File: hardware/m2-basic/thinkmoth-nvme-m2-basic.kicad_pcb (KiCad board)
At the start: 4 copper layers, 31 x 68.4 mm, 24 parts, among them J1 ExpressCard, J2 MDT180M03001, J3 TF-001B, U1 GL823K-HCY04

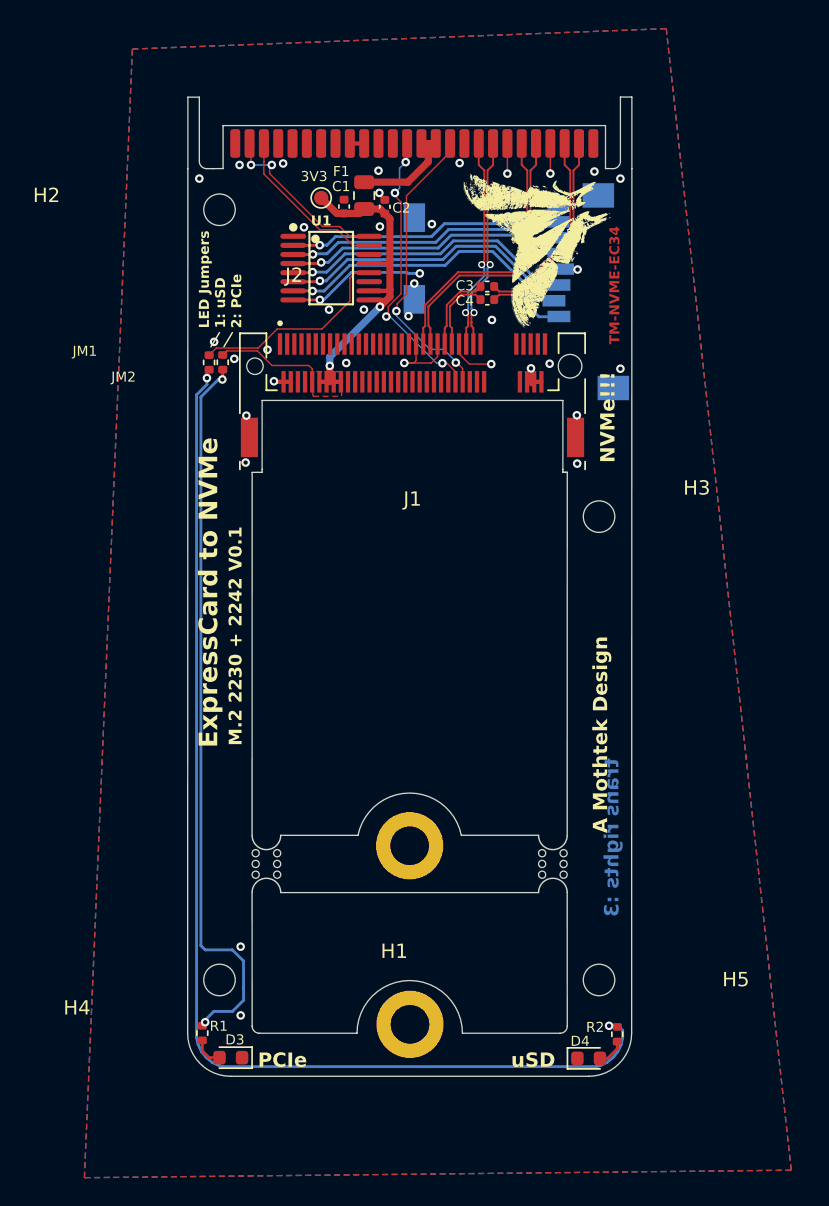
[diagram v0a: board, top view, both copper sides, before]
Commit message: minor tweaks
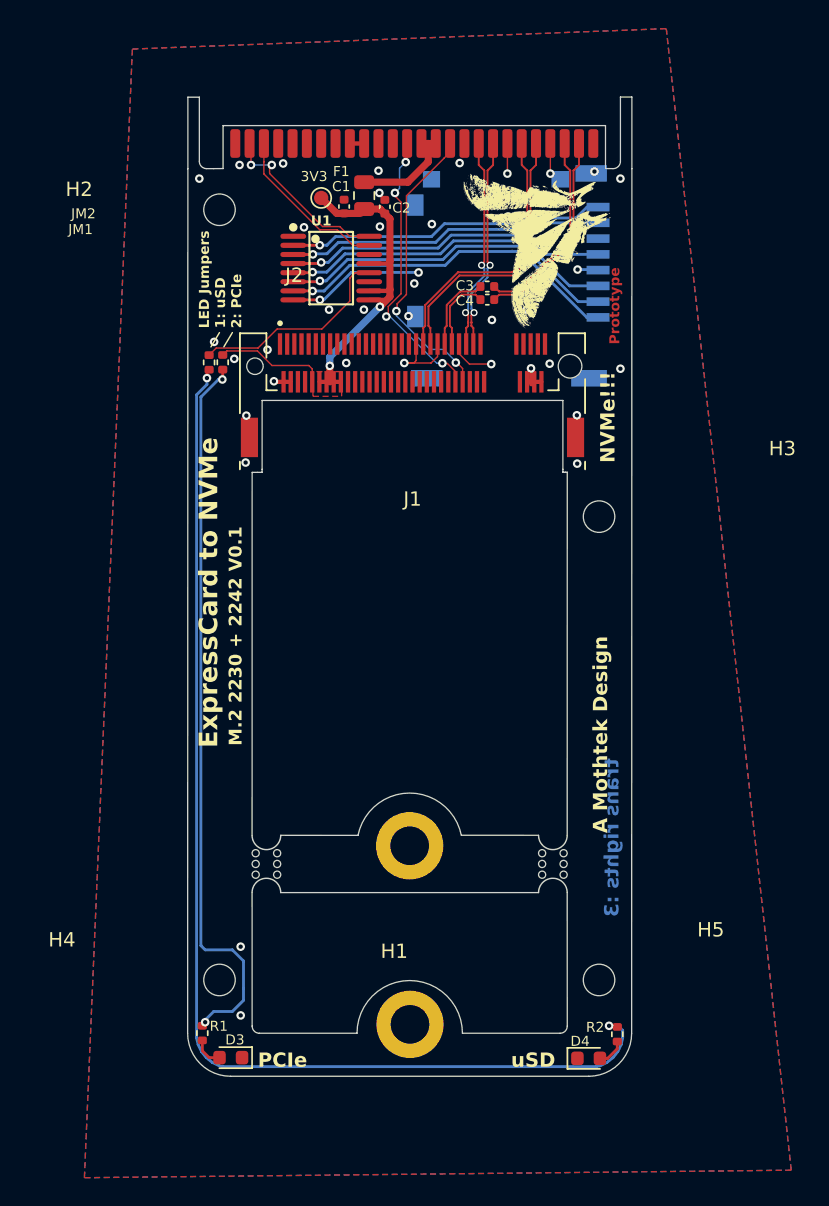
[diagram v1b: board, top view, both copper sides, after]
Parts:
- J3: value TF-001B -> TF-009; footprint SOFNG-TF-001B:TF-SMD_TF-001B -> SOFNG-TF-009:TF-SMD_TF-009
- moved J3 1.22 mm to (82.5, 61.7), turned to 90 degrees
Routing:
- net SD_DAT3: track 20.8 -> 23.9 mm
- net SD_CLK: track 19.9 -> 22.7 mm
- net SD_CMD: track 20.7 -> 23.5 mm
- net SD_DAT1: track 19.7 -> 22.4 mm
- net SD_DAT0: track 19.6 -> 22.3 mm
- net SD_DAT2: track 22.4 -> 24.3 mm
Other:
- board text added: "Prototype"
- board text added: "huge thanks to: wificable 0xarya ambraglow HackMods!!! everyone else :3"
- board text removed: "TM-NVME-EC34"
- board text removed: "huge thanks to: wificable 0xarya ambraglow HackMods everyone else :3"
